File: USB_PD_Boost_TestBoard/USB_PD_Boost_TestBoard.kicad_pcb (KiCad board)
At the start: 2 copper layers, 83.6 x 68.1 mm, 101 parts, among them IC1 CYPD3177-24LQXQ, IC2 TPS55340PWP, J1 USB_C_Receptacle_USB2.0_16P, J2 PD_I2C, J3 575-4, J4 575-4, J5 575-4, J6 575-4, Q1 SI7997DP-T1-GE3, Q2 SI7997DP-T1-GE3, Q3 IRLML0030

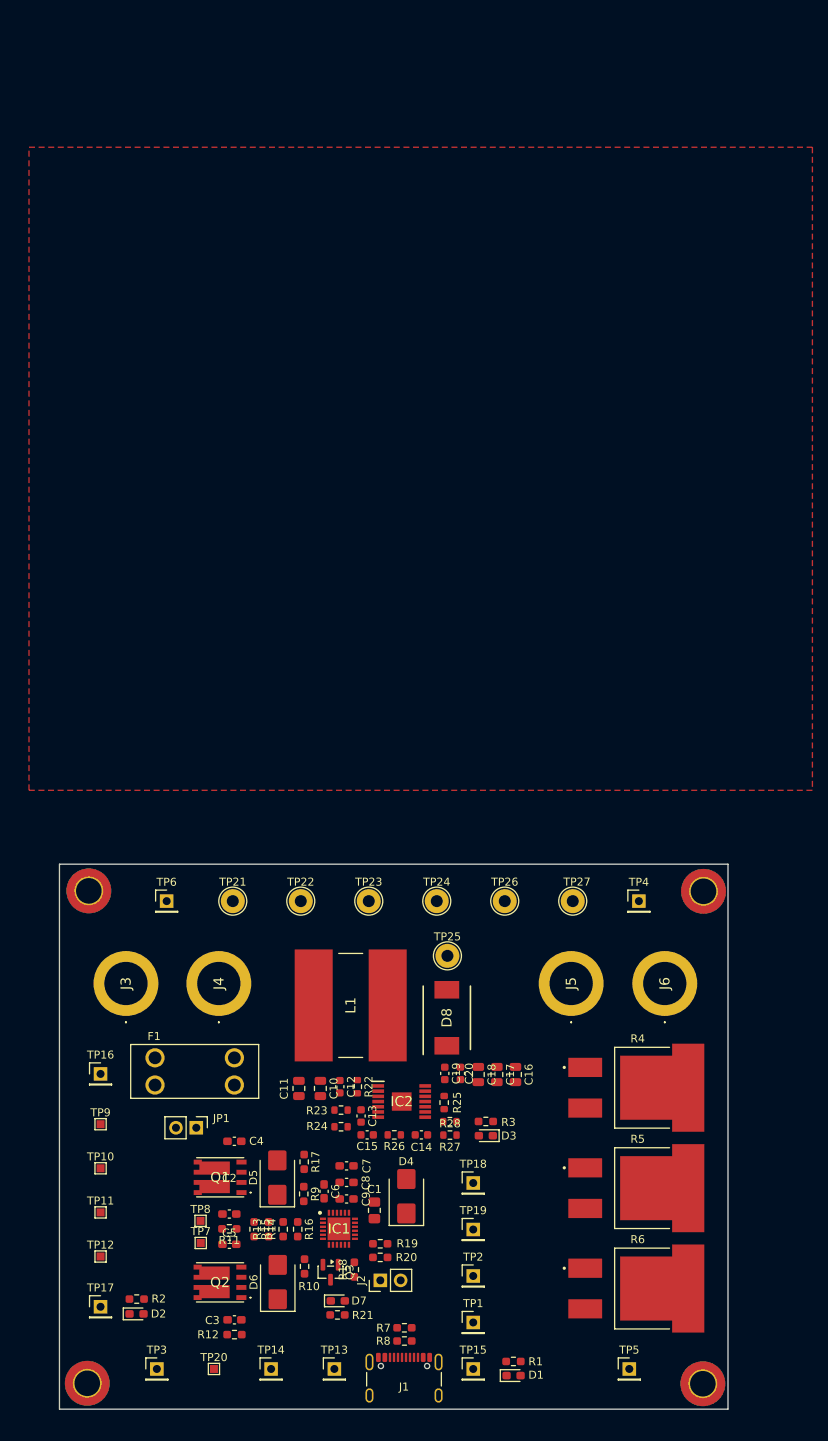
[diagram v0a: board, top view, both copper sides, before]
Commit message: early layout stuff
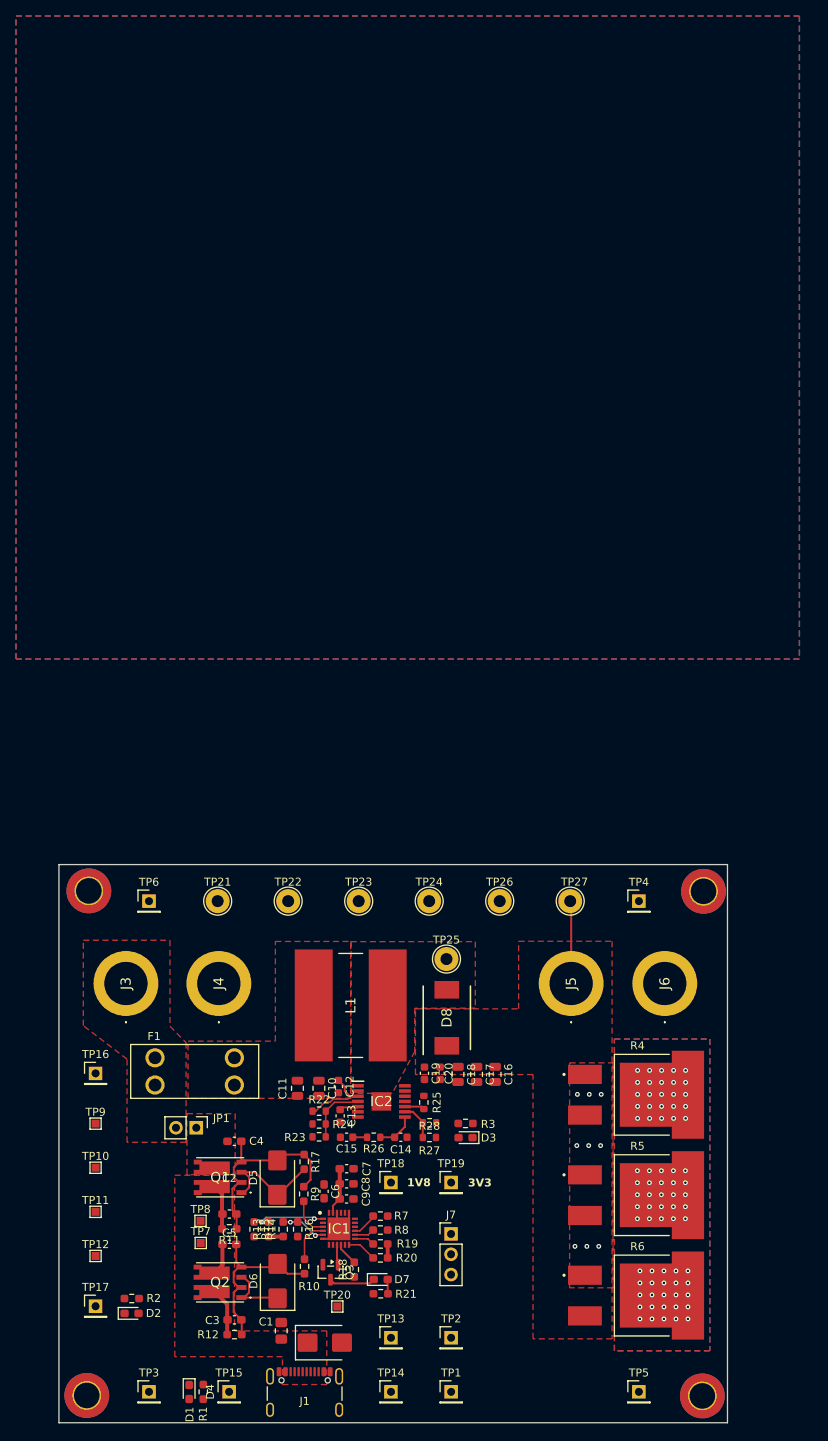
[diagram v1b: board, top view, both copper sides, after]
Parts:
- removed J2: PD_I2C, Connector_PinHeader_2.54mm:PinHeader_1x02_P2.54mm_Vertical
- added J7: PD_12C, Connector_PinHeader_2.54mm:PinHeader_1x03_P2.54mm_Vertical, F.Cu at (142.9, 125.0)
- moved D1 40.6 mm to (110.1, 144.7), turned to -90 degrees
- moved R1 39.0 mm to (111.9, 144.7), turned to -90 degrees
- moved TP15 30.6 mm to (115.1, 144.7)
- moved D4 21.0 mm to (127.1, 138.6), turned to 0 degrees
- moved C1 19.0 mm to (121.6, 137.1)
- moved TP20 17.3 mm to (128.7, 134.1)
- moved TP14 15.3 mm to (135.4, 144.7)
- moved R7 14.3 mm to (134.0, 122.8), turned to 0 degrees
- moved R8 14.2 mm to (134.0, 124.5), turned to 0 degrees
- moved J1 12.6 mm to (124.6, 145.9)
- moved TP18 10.3 mm to (135.4, 118.6)
- moved TP1 9.10 mm to (142.9, 144.7)
- moved TP2 8.20 mm to (142.9, 138.0)
- moved TP13 8.08 mm to (135.4, 138.0)
- moved TP19 6.49 mm to (142.9, 118.6)
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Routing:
- net Net-(D5-A): track 0.00 -> 25.9 mm
- net Net-(D6-A): track 0.00 -> 22.0 mm
- net Net-(D5-K): track 0.00 -> 14.0 mm
- net /VBUS_IN: track 0.00 -> 11.7 mm
- net /BOOST_24V_OUT: track 0.00 -> 10.3 mm
- net /USB_PD_Boost/+USB_PD: track 0.00 -> 10.0 mm
- net /USB_PD/VBUS_MIN: track 0.00 -> 9.83 mm, vias 0 -> 2
- net /USB_PD/PD_3V3: track 0.00 -> 9.42 mm
- net Net-(D6-K): track 0.00 -> 8.28 mm
- net Net-(IC2-EN): track 0.00 -> 7.73 mm
- net GND: track 0.00 -> 7.14 mm, vias 0 -> 9
- net /USB_PD/ISINK_COARSE: track 0.00 -> 6.62 mm, vias 0 -> 2
- net Net-(D7-K): track 0.00 -> 5.79 mm
- net /USB_PD/SAFE_PWR_EN: track 0.00 -> 5.25 mm
- net /USB_PD/VBUS_FET_EN: track 0.00 -> 4.97 mm
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- added copper zone on F.Cu, net /BOOST_24V_OUT
- added copper zone on F.Cu, net /BOOST_VIN
- added copper zone on B.Cu, net /DISSIPATION
- added copper zone on F.Cu, net /DISSIPATION
- added copper zone on F.Cu, net /PD_VOUT
- added copper zone on F.Cu, net /USB_PD_Boost/+USB_PD
- added copper zone on F.Cu, net /VBUS_IN
- added copper zone on B.Cu, net GND
- added copper zone on F.Cu, net Net-(D8-A)
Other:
- board size 83.6 x 68.1 mm -> 83.6 x 69.8 mm
- board text added: "1V8"
- board text added: "3V3"
